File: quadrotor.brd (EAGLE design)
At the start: 45.3 x 45.3 mm, 42 parts, among them T1 AO3400, T2 AO3400, T3 AO3400, T4 AO3400, X1 16MHZ

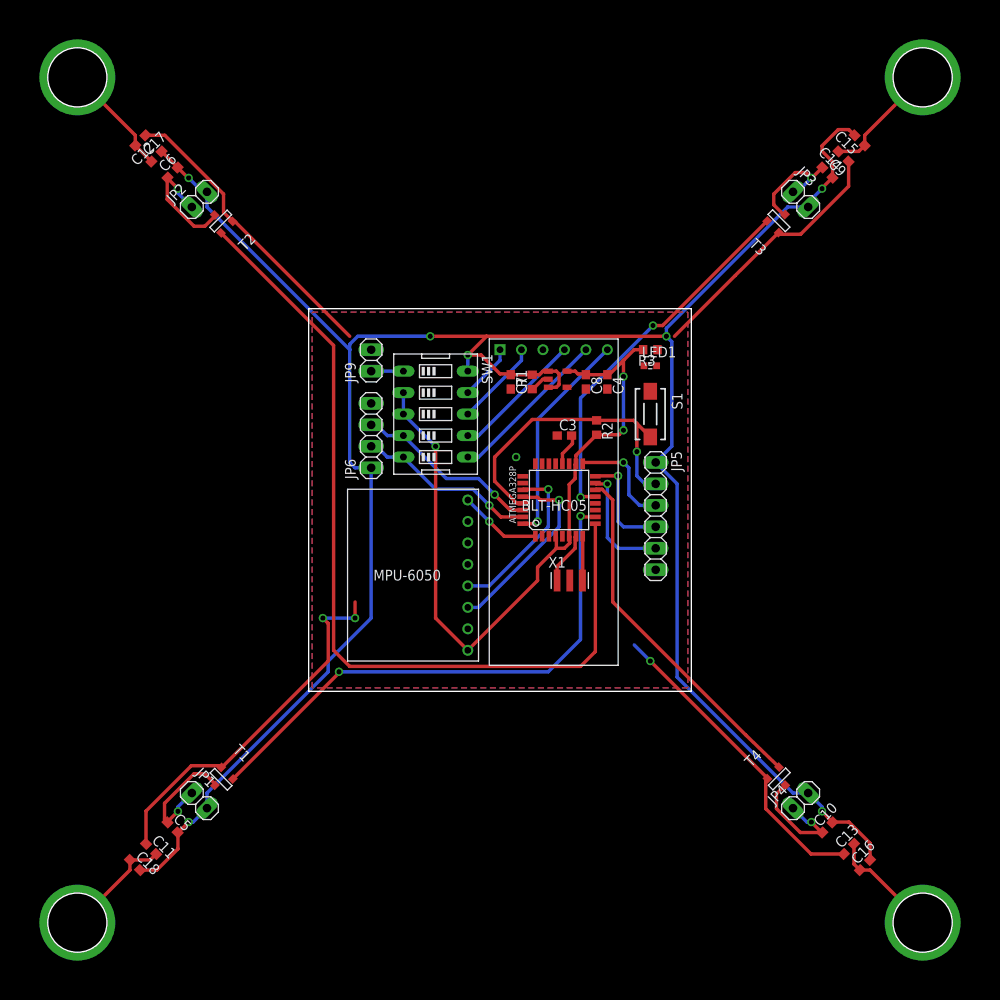
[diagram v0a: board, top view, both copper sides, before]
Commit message: basically done v1 brd
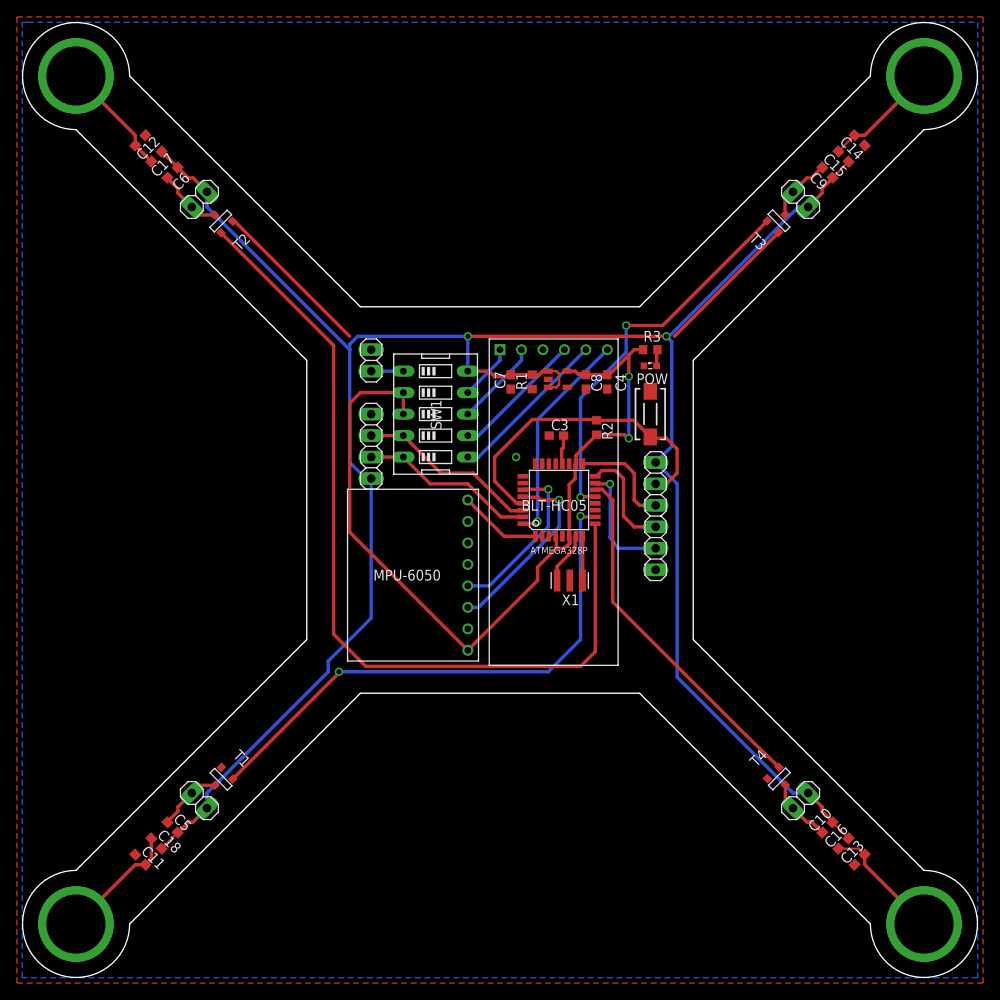
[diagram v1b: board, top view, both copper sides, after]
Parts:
- moved C16 3.59 mm to (40.6, -40.6)
- moved C18 3.59 mm to (-40.6, -40.6)
- moved C14 2.69 mm to (42.5, 42.5)
- moved C15 2.69 mm to (40.6, 40.6), turned to 315 degrees
- moved C11 1.80 mm to (-42.5, -42.5)
- moved C13 1.80 mm to (42.5, -42.5)
- moved JP6 1.27 mm to (-15.2, 6.35)
- moved C3 0.95 mm to (6.67, 7.62)
- moved U$3 0.23 mm to (-50.2, -50.2)
- moved U$4 0.23 mm to (-50.2, 50.2)
- moved U$5 0.23 mm to (50.2, 50.2)
- moved U$6 0.23 mm to (50.2, -50.2)
- renumbered LED1 to POW
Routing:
- net GND: track 150.2 -> 36.9 mm, vias 4 -> 1
- net VIN: track 281.1 -> 262.3 mm, vias 7 -> 2
- net VCC: track 89.6 -> 102.5 mm, vias 3 -> 2
- net N$4: track 15.1 -> 7.78 mm, vias 1 -> 0
- net N$6: track 14.8 -> 7.76 mm, vias 1 -> 0
- net N$9: track 14.5 -> 7.78 mm, vias 1 -> 0
- net N$10: track 13.5 -> 7.76 mm, vias 1 -> 0
- net N$8: track 0.00 -> 1.95 mm
- net M3: track 44.3 -> 46.1 mm
- net N$16: track 13.4 -> 14.5 mm
- net N$5: track 13.4 -> 14.5 mm
- net M2: track 102.5 -> 101.4 mm
- net RESET: track 37.2 -> 38.1 mm, vias 1 -> 0
- net PD1/TX: track 21.4 -> 20.9 mm, vias 1 -> 0
- net PD0/RX: track 22.1 -> 21.6 mm, vias 1 -> 0
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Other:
- board size 45.3 x 45.3 mm -> 113 x 113 mm
